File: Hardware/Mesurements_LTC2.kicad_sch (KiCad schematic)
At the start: 19 parts, among them J11 Conn_01x02, Q2 100V/2W, U2 BQ79614PAPRQ1

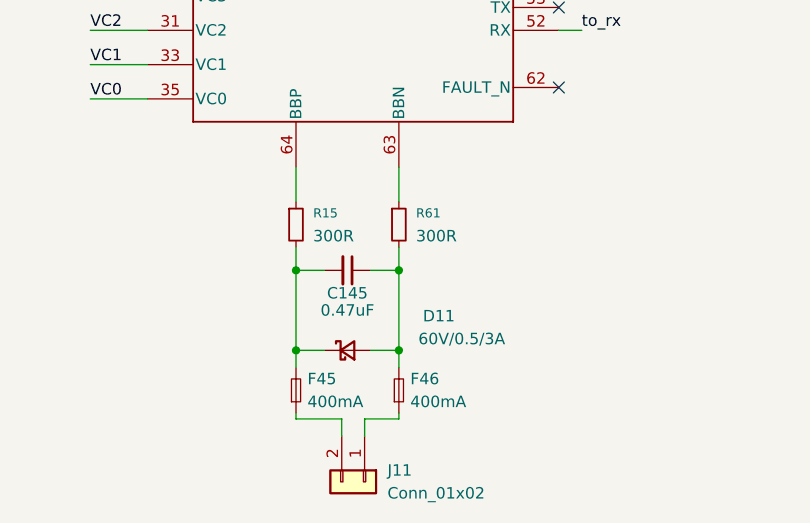
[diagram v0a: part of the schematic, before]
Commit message: No drc errors
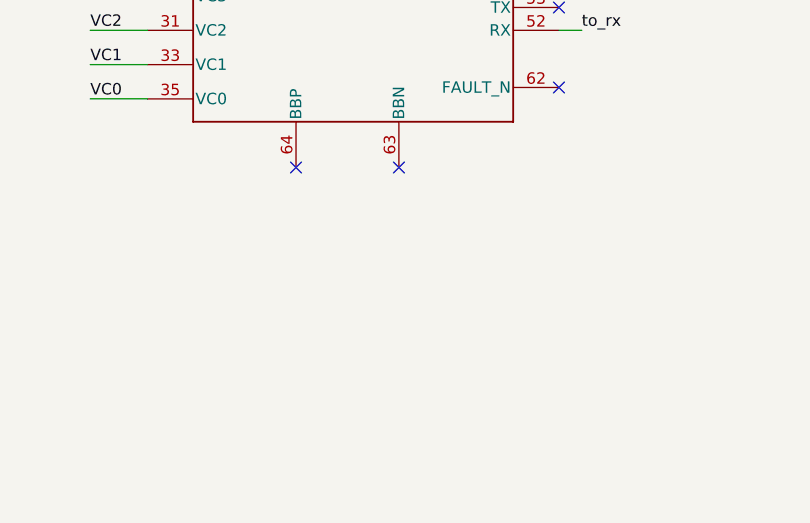
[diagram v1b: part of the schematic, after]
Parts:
- removed C145: 0.47uF, Capacitor_SMD:C_0603_1608Metric_Pad1.08x0.95mm_HandSolder, symbol Device:C_Small
- removed D11: 60V/0.5/3A, Diode_SMD:D_SOD-123, symbol Device:D_Schottky_Small
- removed F45, F46: 400mA, Fuse:Fuse_0805_2012Metric, symbol Device:Fuse_Small
- removed J11: Conn_01x02, Connector_JST:JST_XH_S2B-XH-A_1x02_P2.50mm_Horizontal, symbol Connector_Generic:Conn_01x02
- removed R15, R61: 300R, Resistor_SMD:R_0603_1608Metric, symbol Device:R_Small
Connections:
- no-connect marks 7 -> 9
